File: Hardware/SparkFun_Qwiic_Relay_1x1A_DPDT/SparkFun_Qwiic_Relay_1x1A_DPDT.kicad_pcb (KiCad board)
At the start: 2 copper layers, 25.4 x 33.3 mm, 72 parts, among them J1 Qwiic_RA, J2 Conn_01x03, J3 Qwiic_RA, J4 Conn_01x01, J5 I2C, J6 3.5mm, K2 G6K-2F-Y DC3, Q2 LMUN2235LT1G, U1 PCA9536DP, U3 EL3H7

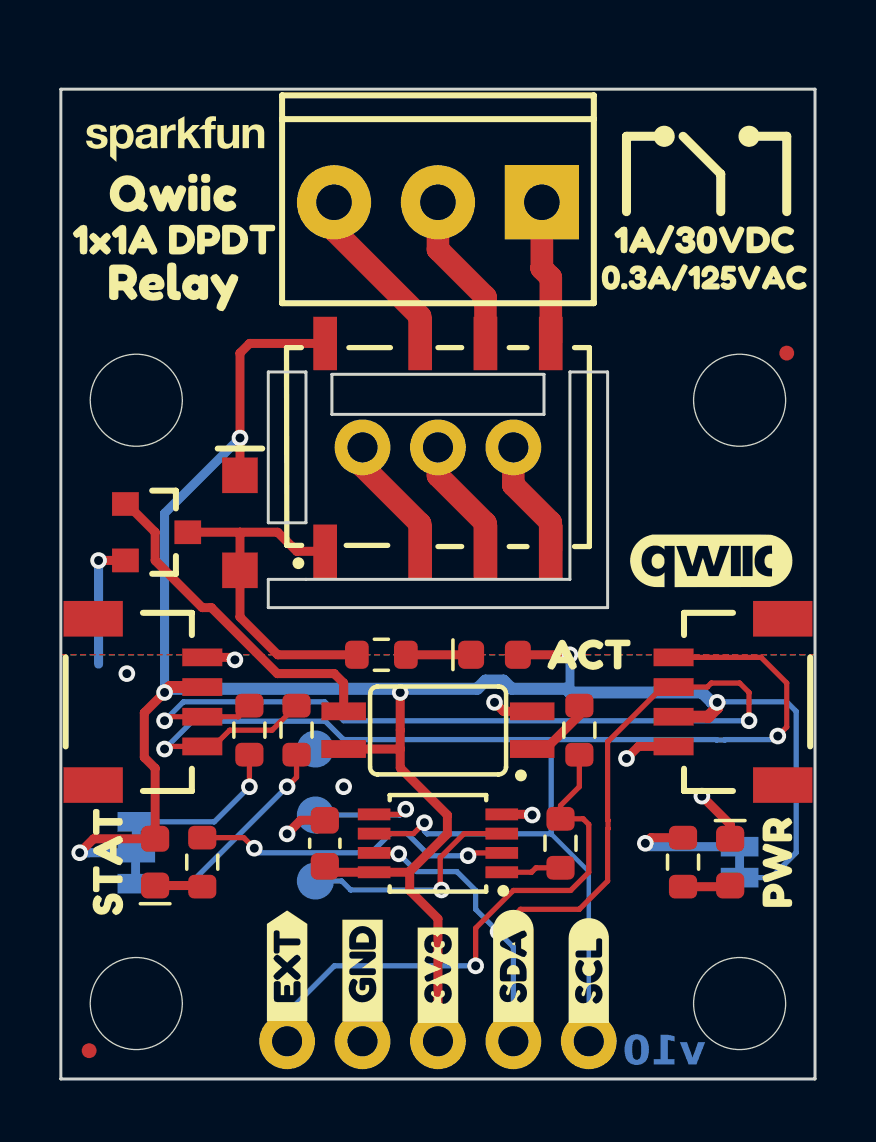
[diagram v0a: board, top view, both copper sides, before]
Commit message: Post review update
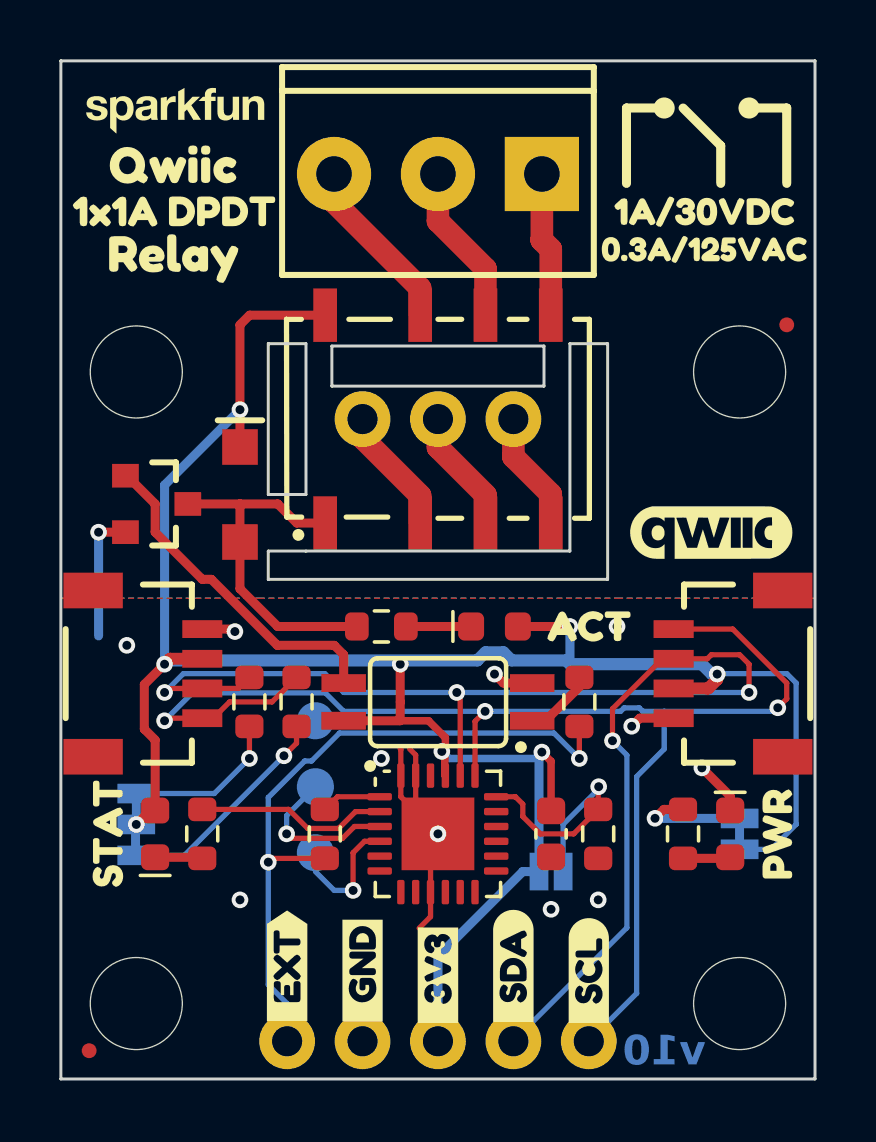
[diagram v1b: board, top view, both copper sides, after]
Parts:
- removed U1: PCA9536DP, SparkFun-Semiconductor-Standard:TSSOP-8_3x3mm_P0.65mm
- added JP1: ADR, SparkFun-Jumper:Jumper_2_NO, B.Cu at (151.8, 110.5)
- added R3: 10k, SparkFun-Resistor:R_0603_1608Metric, F.Cu at (153.4, 109.2)
- added U2: TCA9555RTWR, SparkFun-Semiconductor-Standard:QFN-24-1EP_4x4mm_P0.5mm_EP2.45x2.45mm, F.Cu at (148.0, 109.2)
- added kibuzzard-695DDFCB: G***, kibuzzard-695DDFCB, B.Cu at (154.8, 110.5)
- JP4: value ~ -> LED
- moved Ref** 14.9 mm to (140.3, 112.4)
- moved R2 7.94 mm to (144.1, 109.2), turned to -90 degrees
- moved C1 7.63 mm to (151.8, 109.2), turned to -90 degrees
- moved TP1 3.18 mm to (143.8, 107.6)
- moved TP2 1.27 mm to (143.8, 109.9)
- moved kibuzzard-693716F7 0.95 mm to (148.0, 107.3)
- moved D1 0.95 mm to (157.8, 109.2)
- moved D3 0.95 mm to (138.4, 109.2)
- moved D6 0.95 mm to (149.9, 102.2)
- moved D7 0.95 mm to (141.3, 97.8)
- moved FID4 0.95 mm to (159.7, 92.1)
- moved G*** 0.95 mm to (157.2, 99.1)
- moved G*** 0.95 mm to (139.1, 84.8)
- moved G*** 0.95 mm to (148.0, 103.8)
- moved J1 0.95 mm to (155.9, 103.8)
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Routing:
- net Net-(JP1-A): track 0.00 -> 8.66 mm, vias 0 -> 1
- net GND: track 13.0 -> 20.4 mm, vias 9 -> 12
- net STAT_LED: track 10.9 -> 6.48 mm, vias 2 -> 0
- net Ext_Drive: track 18.9 -> 23.2 mm, vias 1 -> 2
- net SCL: track 49.6 -> 46.5 mm
- net SDA: track 48.6 -> 45.5 mm
- net IO2: track 7.89 -> 5.35 mm
- net 3.3V: track 80.3 -> 82.6 mm, vias 6 -> 8
- net Net-(JP4-A): track 4.57 -> 3.92 mm
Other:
- board size 25.4 x 33.3 mm -> 25.4 x 34.3 mm
